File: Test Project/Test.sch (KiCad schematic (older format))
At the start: 1 part

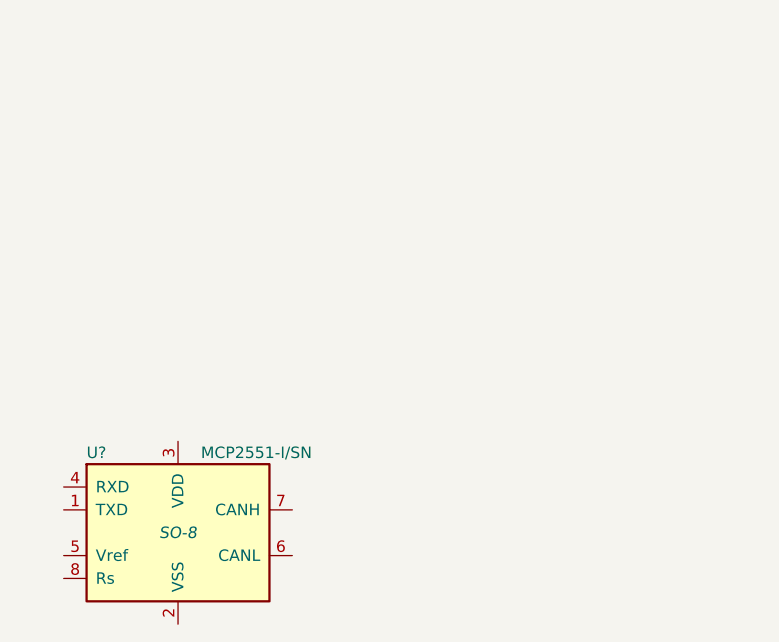
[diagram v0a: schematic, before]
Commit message: Summer
Added very important component layout
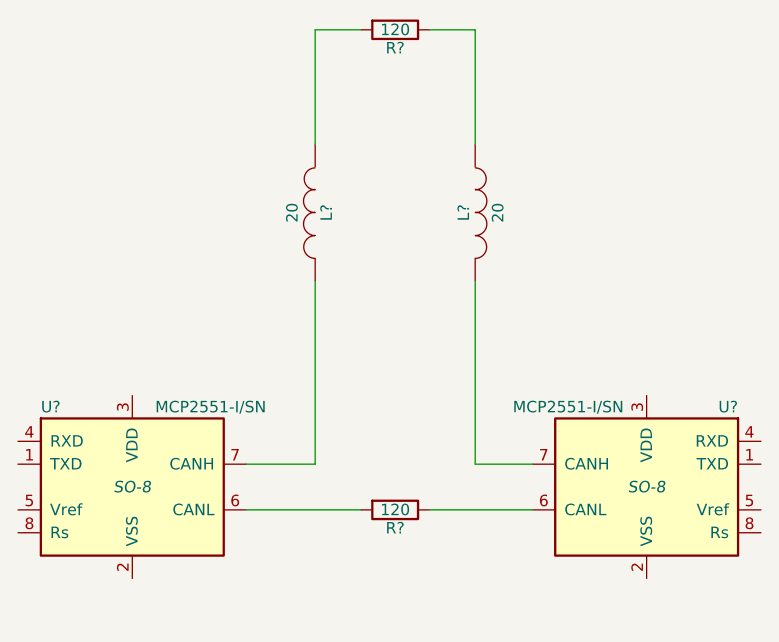
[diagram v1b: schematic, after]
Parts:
- added L? (x2): 20, symbol INDUCTOR
- added R? (x2): 120, symbol R
- added U?: MCP2551-I/SN, SO-8, symbol MCP2551-I/SN
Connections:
- net at U?.6 (CANL): now also R?.2
- net at U?.7 (CANH): now also L?.2
- new net: L?.1, R?.1
- new net: L?.2, U?.7 (CANH)
- new net: R?.1, U?.6 (CANL)
- new net: L?.1, R?.2
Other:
- moved on the sheet: U?
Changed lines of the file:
@@
 LIBS:memory
 LIBS:xilinx
-LIBS:special
 LIBS:microcontrollers
 LIBS:dsp
@@
 L MCP2551-I/SN U?
 U 1 1 559C6BBA
-P 4800 3800
-F 0 "U?" H 4400 4150 50  0000 L CNN
-F 1 "MCP2551-I/SN" H 4900 4150 50  0000 L CNN
-F 2 "SO-8" H 4800 3800 50  0000 C CIN
-F 3 "" H 4800 3800 60  0000 C CNN
-	1    4800 3800
+P 4600 3600
+F 0 "U?" H 4200 3950 50  0000 L CNN
+F 1 "MCP2551-I/SN" H 4700 3950 50  0000 L CNN
+F 2 "SO-8" H 4600 3600 50  0000 C CIN
+F 3 "" H 4600 3600 60  0000 C CNN
+	1    4600 3600
 	1    0    0    -1
 $EndComp
+$Comp
+L INDUCTOR L?
+U 1 1 559DCECC
+P 6100 2400
+F 0 "L?" V 6050 2400 50  0000 C CNN
+F 1 "20" V 6200 2400 50  0000 C CNN
+F 2 "" H 6100 2400 60  0000 C CNN
+F 3 "" H 6100 2400 60  0000 C CNN
+	1    6100 2400
+	1    0    0    -1
+$EndComp
+$Comp
+L MCP2551-I/SN U?
+U 1 1 559DD087
+P 6850 3600
+F 0 "U?" H 6450 3950 50  0000 L CNN
+F 1 "MCP2551-I/SN" H 6950 3950 50  0000 L CNN
+F 2 "SO-8" H 6850 3600 50  0000 C CIN
+F 3 "" H 6850 3600 60  0000 C CNN
+	1    6850 3600
+	-1   0    0    -1
+$EndComp
+$Comp
+L INDUCTOR L?
+U 1 1 559DD128
+P 5400 2400
+F 0 "L?" V 5350 2400 50  0000 C CNN
+F 1 "20" V 5500 2400 50  0000 C CNN
+F 2 "" H 5400 2400 60  0000 C CNN
+F 3 "" H 5400 2400 60  0000 C CNN
+	1    5400 2400
+	-1   0    0    -1
+$EndComp
+Wire Wire Line
+	5400 2700 5400 3500
+Wire Wire Line
+	5400 3500 5100 3500
+$Comp
+L R R?
+U 1 1 559DD2E2
+P 5750 1600
+F 0 "R?" V 5830 1600 50  0000 C CNN
+F 1 "120" V 5750 1600 50  0000 C CNN
+F 2 "" V 5680 1600 30  0000 C CNN
+F 3 "" H 5750 1600 30  0000 C CNN
+	1    5750 1600
+	0    1    1    0
+$EndComp
+$Comp
+L R R?
+U 1 1 559DD3B4
+P 5750 3700
+F 0 "R?" V 5830 3700 50  0000 C CNN
+F 1 "120" V 5750 3700 50  0000 C CNN
+F 2 "" V 5680 3700 30  0000 C CNN
+F 3 "" H 5750 3700 30  0000 C CNN
+	1    5750 3700
+	0    1    1    0
+$EndComp
+Wire Wire Line
+	5400 1600 5600 1600
+Wire Wire Line
+	5900 1600 6100 1600
+Wire Wire Line
+	5400 2100 5400 1600
+Wire Wire Line
+	6100 1600 6100 2100
+Wire Wire Line
+	6100 2700 6100 3500
+Wire Wire Line
+	6100 3500 6350 3500
+Wire Wire Line
+	5900 3700 6350 3700
+Wire Wire Line
+	5600 3700 5100 3700
 $EndSCHEMATC
